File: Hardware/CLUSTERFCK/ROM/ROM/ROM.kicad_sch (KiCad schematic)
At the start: 39 parts, among them SW3 SW_DIP_x02, U30 28c64, U31 28c64

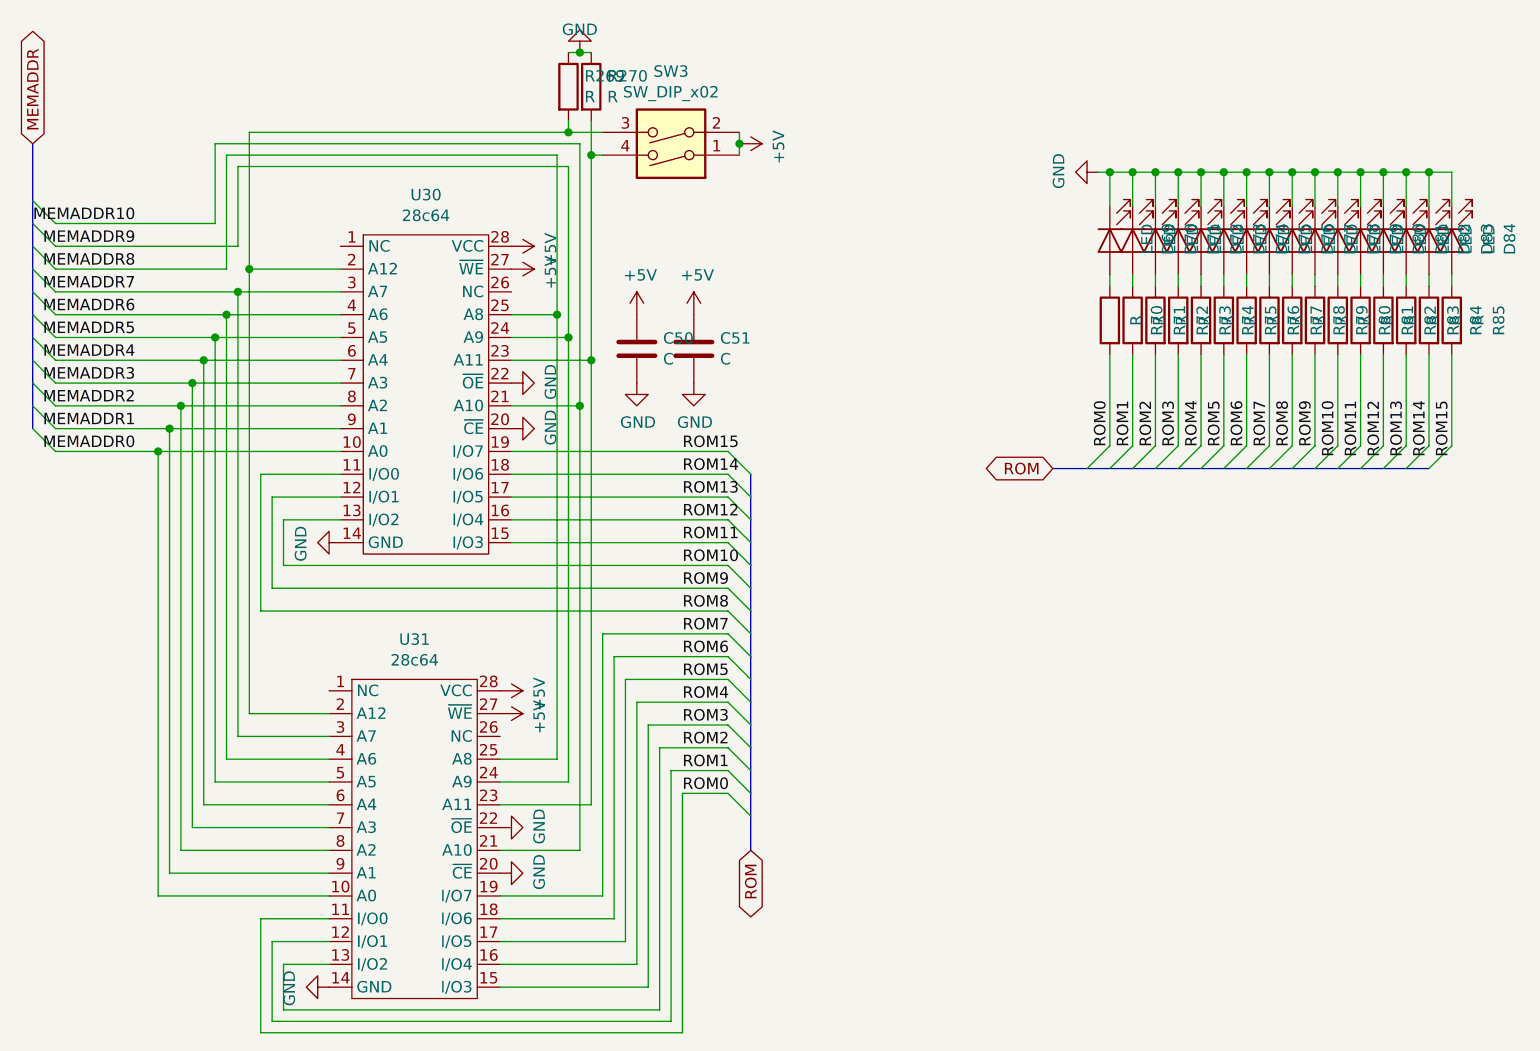
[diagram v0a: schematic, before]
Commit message: 0031 | 10h | PCB MARMEM
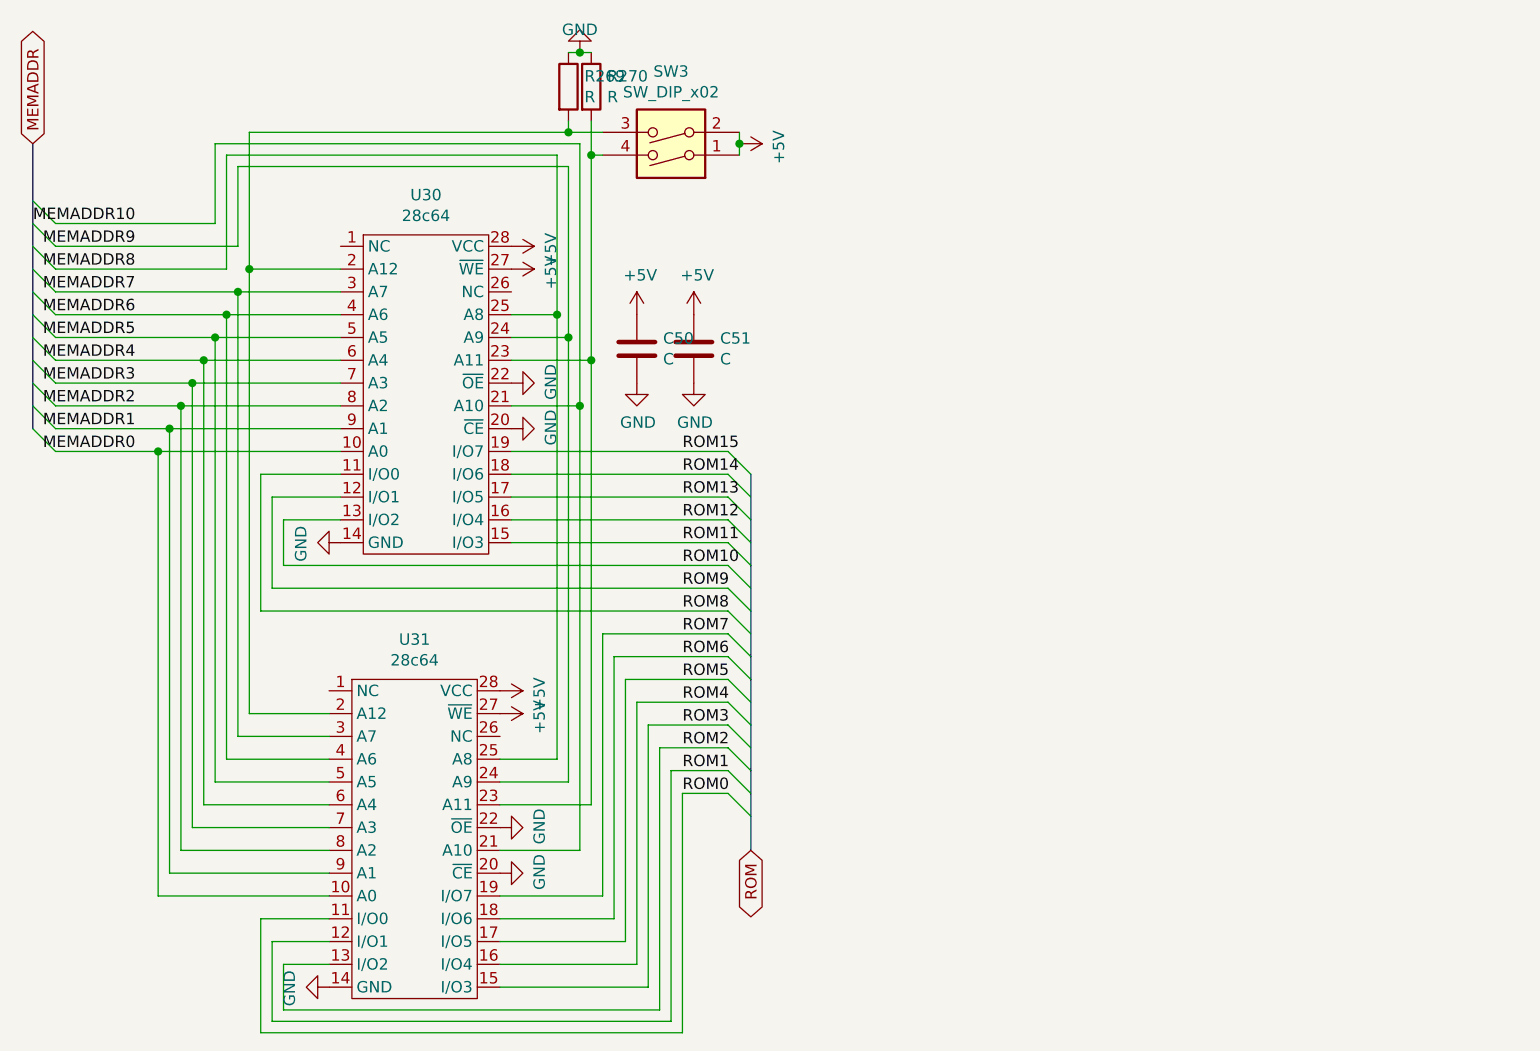
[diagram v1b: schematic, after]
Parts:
- removed D69, D70, D71, D72, D73, D74, D75, D76, D77, D78, D79, D80, D81, D82, D83, D84: LED, LED_THT:LED_D5.0mm, symbol Device:LED
- removed R70, R71, R72, R73, R74, R75, R76, R77, R78, R79, R80, R81, R82, R83, R84, R85: R, Resistor_SMD:R_0805_2012Metric_Pad1.15x1.40mm_HandSolder, symbol Device:R
